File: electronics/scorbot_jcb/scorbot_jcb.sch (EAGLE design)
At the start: 5 parts

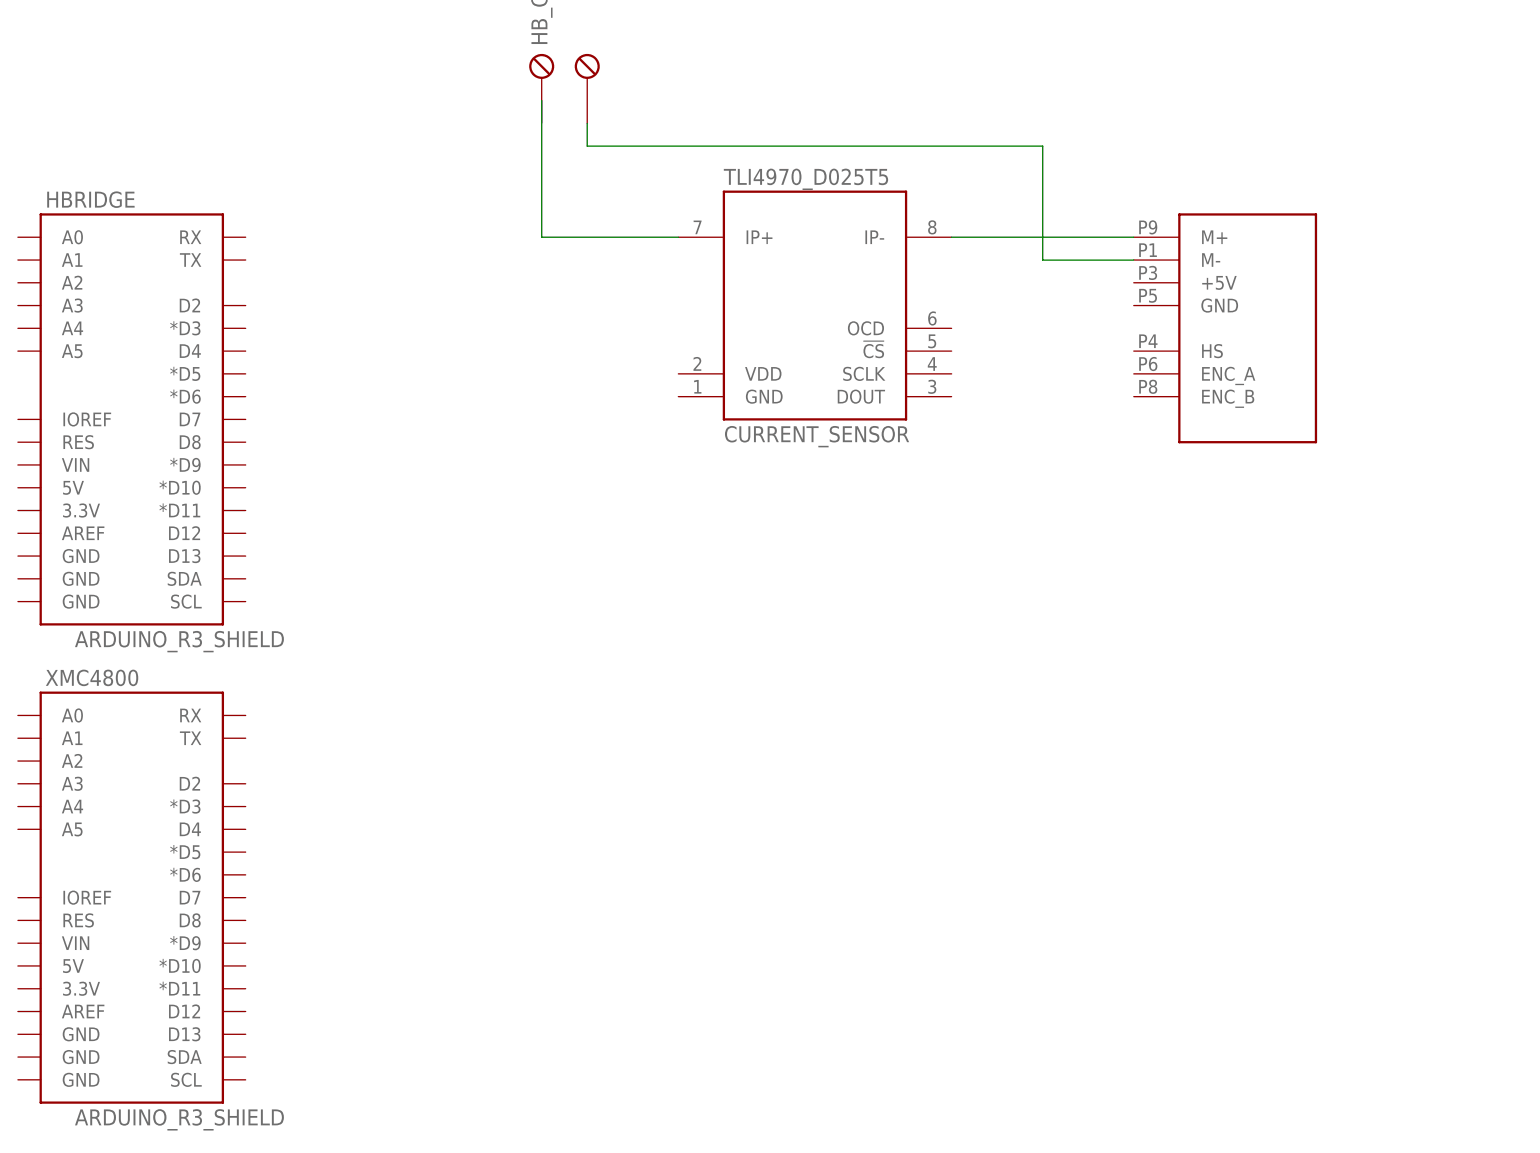
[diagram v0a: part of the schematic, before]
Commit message: Current sensor
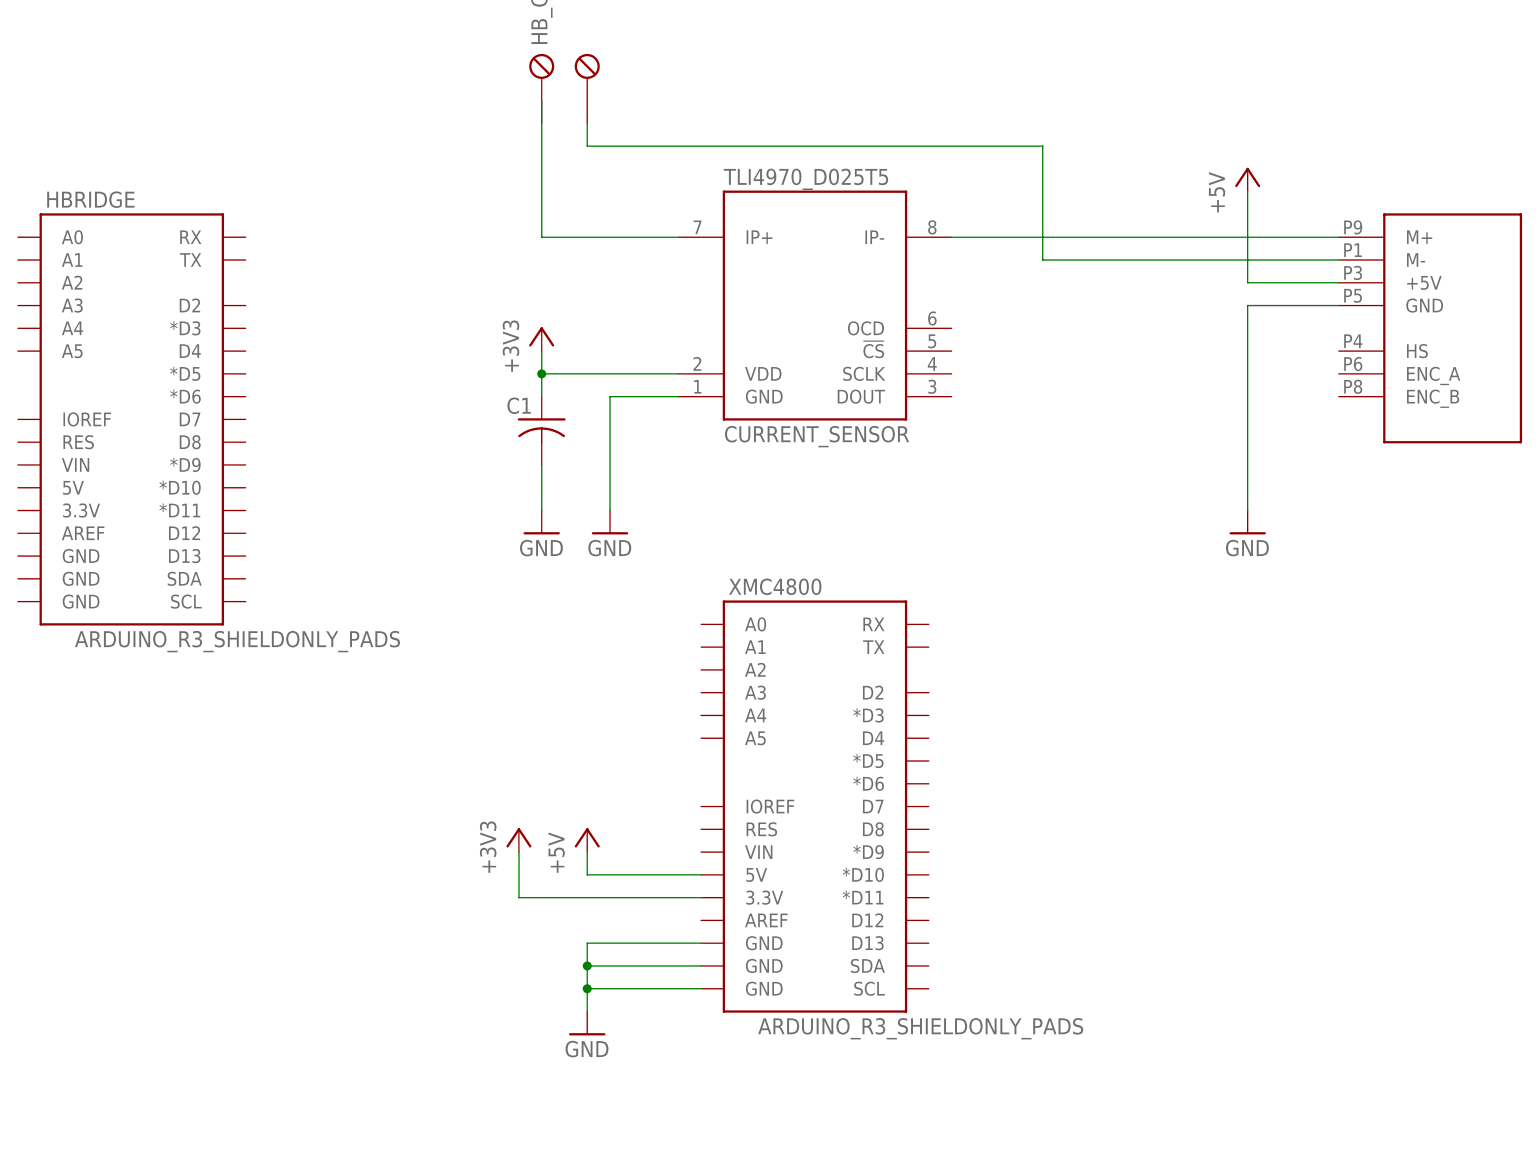
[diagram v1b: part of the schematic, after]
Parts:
- added C1: (no value), rcl:C-US025-025X050
- HBRIDGE, XMC4800: value ARDUINO_R3_SHIELD -> ARDUINO_R3_SHIELDONLY_PADS; device uchile_robotics_eagle_lib:ARDUINO_R3_SHIELD -> uchile_robotics_eagle_lib:ARDUINO_R3_SHIELDONLY_PADS
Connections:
- new net +3V3: C1.1, CURRENT_SENSOR.VDD, XMC4800.3.3V
- new net +5V: DB9.+5V, XMC4800.5V
- new net GND: C1.2, CURRENT_SENSOR.GND, DB9.GND, XMC4800.GND@0, XMC4800.GND@1, XMC4800.GND@2
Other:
- moved on the sheet: XMC4800
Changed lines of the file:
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@@
 <setting verticaltext="up"/>
 </settings>
-<grid distance="0.1" unitdist="inch" unit="inch" style="lines" multiple="1" display="yes" altdistance="0.01" altunitdist="inch" altunit="inch"/>
+<grid distance="0.1" unitdist="inch" unit="inch" style="lines" multiple="1" display="no" altdistance="0.01" altunitdist="inch" altunit="inch"/>
 <layers>
 <layer number="1" name="Top" color="4" fill="1" visible="no" active="no"/>
@@
 <part name="DB9" library="uchile_robotics_eagle_lib" deviceset="SCORBOT_CONNECTOR" device=""/>
 <part name="CURRENT_SENSOR" library="uchile_robotics_eagle_lib" deviceset="TLI4970_D025T5" device=""/>
-<part name="HBRIDGE" library="uchile_robotics_eagle_lib" deviceset="ARDUINO_R3_SHIELD" device=""/>
-<part name="XMC4800" library="uchile_robotics_eagle_lib" deviceset="ARDUINO_R3_SHIELD" device=""/>
+<part name="HBRIDGE" library="uchile_robotics_eagle_lib" deviceset="ARDUINO_R3_SHIELD" device="ONLY_PADS" value="ARDUINO_R3_SHIELDONLY_PADS"/>
+<part name="XMC4800" library="uchile_robotics_eagle_lib" deviceset="ARDUINO_R3_SHIELD" device="ONLY_PADS" value="ARDUINO_R3_SHIELDONLY_PADS"/>
 <part name="HB_OUT" library="uchile_robotics_eagle_lib" deviceset="METALTEX-2" device="SHORT"/>
+<part name="+3V1" library="supply1" deviceset="+3V3" device=""/>
+<part name="P+1" library="supply1" deviceset="+5V" device=""/>
+<part name="+3V2" library="supply1" deviceset="+3V3" device=""/>
+<part name="GND1" library="supply1" deviceset="GND" device=""/>
+<part name="GND2" library="supply1" deviceset="GND" device=""/>
+<part name="P+2" library="supply1" deviceset="+5V" device=""/>
+<part name="GND3" library="supply1" deviceset="GND" device=""/>
+<part name="C1" library="rcl" deviceset="C-US" device="025-025X050"/>
+<part name="GND4" library="supply1" deviceset="GND" device=""/>
 </parts>
 <sheets>
@@
 </plain>
 <instances>
-<instance part="DB9" gate="G$1" x="144.78" y="76.2"/>
+<instance part="DB9" gate="G$1" x="167.64" y="76.2"/>
 <instance part="CURRENT_SENSOR" gate="G$1" x="96.52" y="78.74" rot="MR180"/>
 <instance part="HBRIDGE" gate="G$1" x="20.32" y="68.58"/>
-<instance part="XMC4800" gate="G$1" x="20.32" y="15.24"/>
+<instance part="XMC4800" gate="G$1" x="96.52" y="25.4"/>
 <instance part="HB_OUT" gate="G$1" x="66.04" y="106.68" rot="R90"/>
+<instance part="+3V1" gate="G$1" x="63.5" y="20.32"/>
+<instance part="P+1" gate="1" x="71.12" y="20.32"/>
+<instance part="+3V2" gate="G$1" x="66.04" y="76.2"/>
+<instance part="GND1" gate="1" x="73.66" y="53.34"/>
+<instance part="GND2" gate="1" x="71.12" y="-2.54"/>
+<instance part="P+2" gate="1" x="144.78" y="93.98"/>
+<instance part="GND3" gate="1" x="144.78" y="53.34"/>
+<instance part="C1" gate="G$1" x="66.04" y="66.04" rot="MR0"/>
+<instance part="GND4" gate="1" x="66.04" y="53.34"/>
 </instances>
 <busses>
@@
 <pinref part="CURRENT_SENSOR" gate="G$1" pin="IP-"/>
 <pinref part="DB9" gate="G$1" pin="M+"/>
-<wire x1="111.76" y1="86.36" x2="132.08" y2="86.36" width="0.1524" layer="91"/>
+<wire x1="111.76" y1="86.36" x2="154.94" y2="86.36" width="0.1524" layer="91"/>
 </segment>
 </net>
@@
 <wire x1="121.92" y1="96.52" x2="121.92" y2="83.82" width="0.1524" layer="91"/>
 <pinref part="DB9" gate="G$1" pin="M-"/>
-<wire x1="121.92" y1="83.82" x2="132.08" y2="83.82" width="0.1524" layer="91"/>
-</segment>
-</net>
+<wire x1="121.92" y1="83.82" x2="154.94" y2="83.82" width="0.1524" layer="91"/>
+</segment>
+</net>
+<net name="+3V3" class="0">
+<segment>
+<pinref part="+3V1" gate="G$1" pin="+3V3"/>
+<wire x1="63.5" y1="17.78" x2="63.5" y2="12.7" width="0.1524" layer="91"/>
+<pinref part="XMC4800" gate="G$1" pin="3.3V"/>
+<wire x1="63.5" y1="12.7" x2="83.82" y2="12.7" width="0.1524" layer="91"/>
+</segment>
+<segment>
+<pinref part="CURRENT_SENSOR" gate="G$1" pin="VDD"/>
+<pinref part="+3V2" gate="G$1" pin="+3V3"/>
+<wire x1="81.28" y1="71.12" x2="66.04" y2="71.12" width="0.1524" layer="91"/>
+<wire x1="66.04" y1="71.12" x2="66.04" y2="73.66" width="0.1524" layer="91"/>
+<pinref part="C1" gate="G$1" pin="1"/>
+<wire x1="66.04" y1="68.58" x2="66.04" y2="71.12" width="0.1524" layer="91"/>
+<junction x="66.04" y="71.12"/>
+</segment>
+</net>
+<net name="+5V" class="0">
+<segment>
+<pinref part="XMC4800" gate="G$1" pin="5V"/>
+<pinref part="P+1" gate="1" pin="+5V"/>
+<wire x1="83.82" y1="15.24" x2="71.12" y2="15.24" width="0.1524" layer="91"/>
+<wire x1="71.12" y1="15.24" x2="71.12" y2="17.78" width="0.1524" layer="91"/>
+</segment>
+<segment>
+<pinref part="DB9" gate="G$1" pin="+5V"/>
+<pinref part="P+2" gate="1" pin="+5V"/>
+<wire x1="154.94" y1="81.28" x2="144.78" y2="81.28" width="0.1524" layer="91"/>
+<wire x1="144.78" y1="81.28" x2="144.78" y2="91.44" width="0.1524" layer="91"/>
+</segment>
+</net>
+<net name="GND" class="0">
+<segment>
+<pinref part="CURRENT_SENSOR" gate="G$1" pin="GND"/>
+<pinref part="GND1" gate="1" pin="GND"/>
+<wire x1="81.28" y1="68.58" x2="73.66" y2="68.58" width="0.1524" layer="91"/>
+<wire x1="73.66" y1="68.58" x2="73.66" y2="55.88" width="0.1524" layer="91"/>
+</segment>
+<segment>
+<pinref part="GND2" gate="1" pin="GND"/>
+<wire x1="71.12" y1="0" x2="71.12" y2="2.54" width="0.1524" layer="91"/>
+<pinref part="XMC4800" gate="G$1" pin="GND@0"/>
+<wire x1="71.12" y1="2.54" x2="83.82" y2="2.54" width="0.1524" layer="91"/>
+<pinref part="XMC4800" gate="G$1" pin="GND@1"/>
+<wire x1="83.82" y1="5.08" x2="71.12" y2="5.08" width="0.1524" layer="91"/>
+<wire x1="71.12" y1="5.08" x2="71.12" y2="2.54" width="0.1524" layer="91"/>
+<pinref part="XMC4800" gate="G$1" pin="GND@2"/>
+<wire x1="83.82" y1="7.62" x2="71.12" y2="7.62" width="0.1524" layer="91"/>
+<wire x1="71.12" y1="7.62" x2="71.12" y2="5.08" width="0.1524" layer="91"/>
+<junction x="71.12" y="5.08"/>
+<junction x="71.12" y="2.54"/>
+</segment>
+<segment>
+<pinref part="GND3" gate="1" pin="GND"/>
+<wire x1="144.78" y1="55.88" x2="144.78" y2="78.74" width="0.1524" layer="91"/>
+<pinref part="DB9" gate="G$1" pin="GND"/>
+<wire x1="144.78" y1="78.74" x2="154.94" y2="78.74" width="0.1524" layer="91"/>
+</segment>
+<segment>
+<pinref part="GND4" gate="1" pin="GND"/>
+<pinref part="C1" gate="G$1" pin="2"/>
+<wire x1="66.04" y1="55.88" x2="66.04" y2="60.96" width="0.1524" layer="91"/>
+</segment>
+</net>

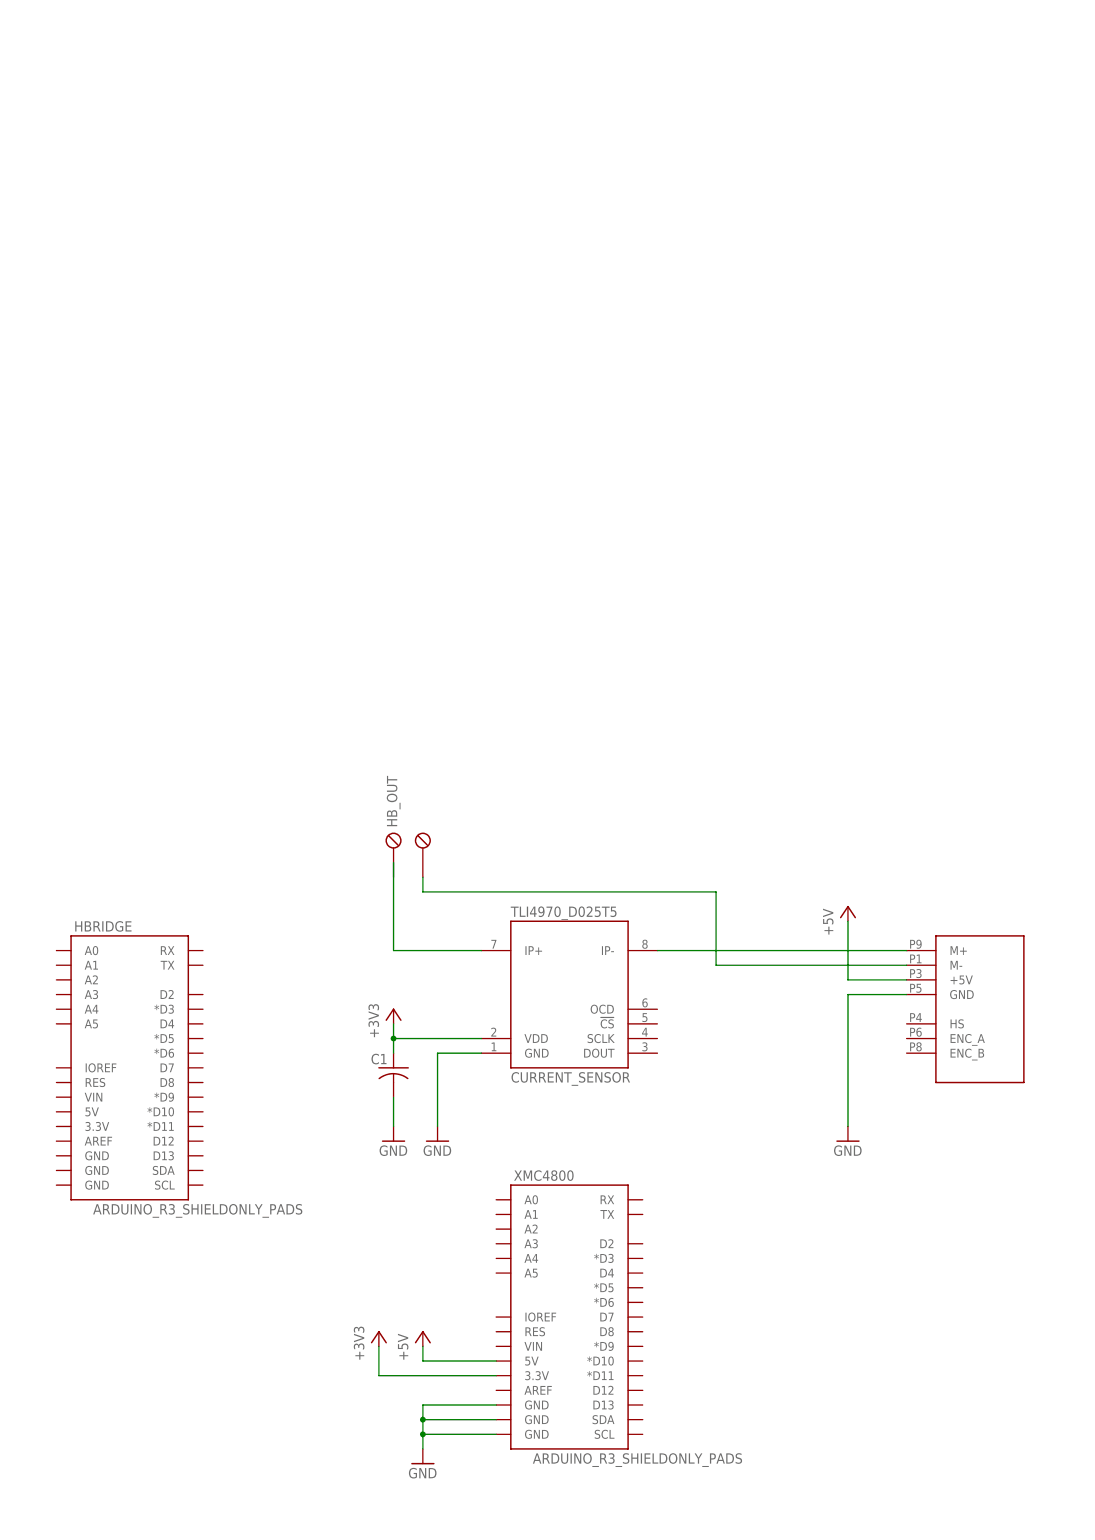
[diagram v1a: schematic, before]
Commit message: Schematic for shield
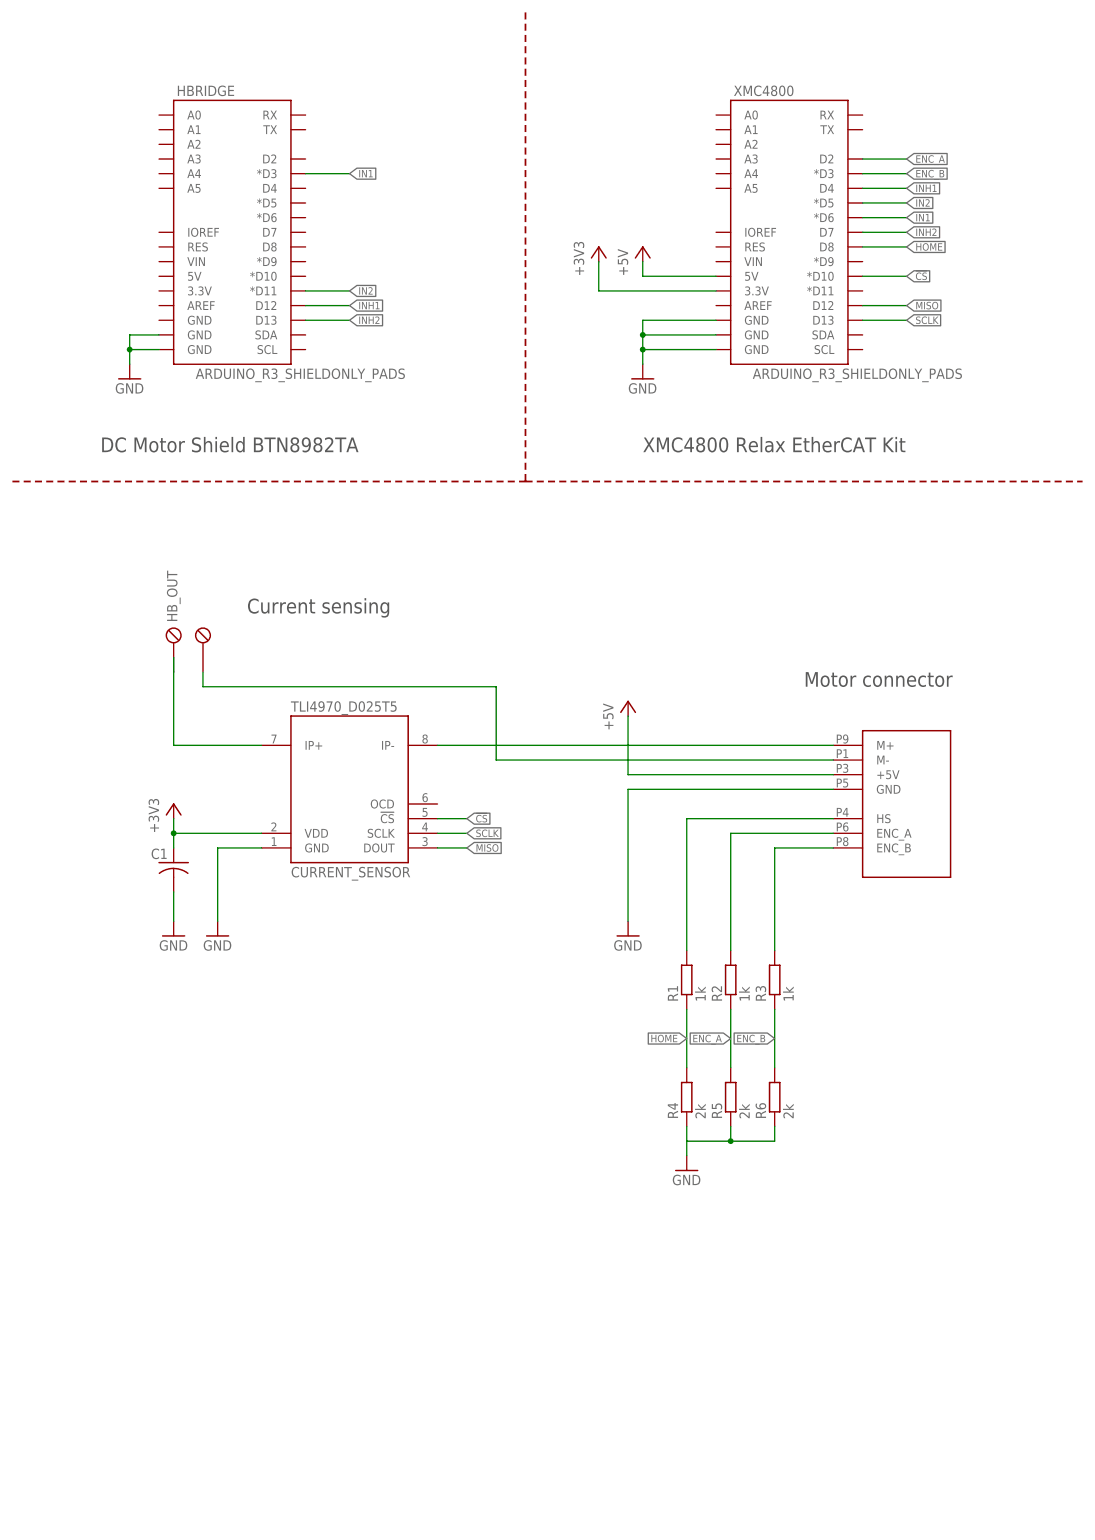
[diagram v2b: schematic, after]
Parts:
- added R1, R2, R3: 1k, rcl:R-EU_0309/12
- added R4, R5, R6: 2k, rcl:R-EU_0309/12
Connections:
- new net !CS: CURRENT_SENSOR.!CS, XMC4800.*D10
- new net ENC_A: R2.1, R5.2, XMC4800.D2
- new net ENC_B: R3.1, R6.2, XMC4800.*D3
- new net HOME: R1.1, R4.2, XMC4800.D8
- new net IN1: HBRIDGE.*D3, XMC4800.*D6
- new net IN2: HBRIDGE.*D11, XMC4800.*D5
- new net INH1: HBRIDGE.D12, XMC4800.D4
- new net INH2: HBRIDGE.D13, XMC4800.D7
- new net MISO: CURRENT_SENSOR.DOUT, XMC4800.D12
- new net N$10: DB9.ENC_A, R2.2
- new net N$11: DB9.ENC_B, R3.2
- new net N$9: DB9.HS, R1.2
- new net SCLK: CURRENT_SENSOR.SCLK, XMC4800.D13
- net GND: now also HBRIDGE.GND@0, HBRIDGE.GND@1, R4.1, R5.1, R6.1
- net N$2: now also HB_OUT.P1
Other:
- note added: "Current sensing"
- note added: "DC Motor Shield BTN8982TA"
- note added: "Motor connector"
- note added: "XMC4800 Relax EtherCAT Kit"
- moved on the sheet: C1, CURRENT_SENSOR, HBRIDGE, HB_OUT, XMC4800
